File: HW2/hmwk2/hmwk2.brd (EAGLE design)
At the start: 50 x 50 mm, 22 parts, among them J1 USB_MINI-B_SMT

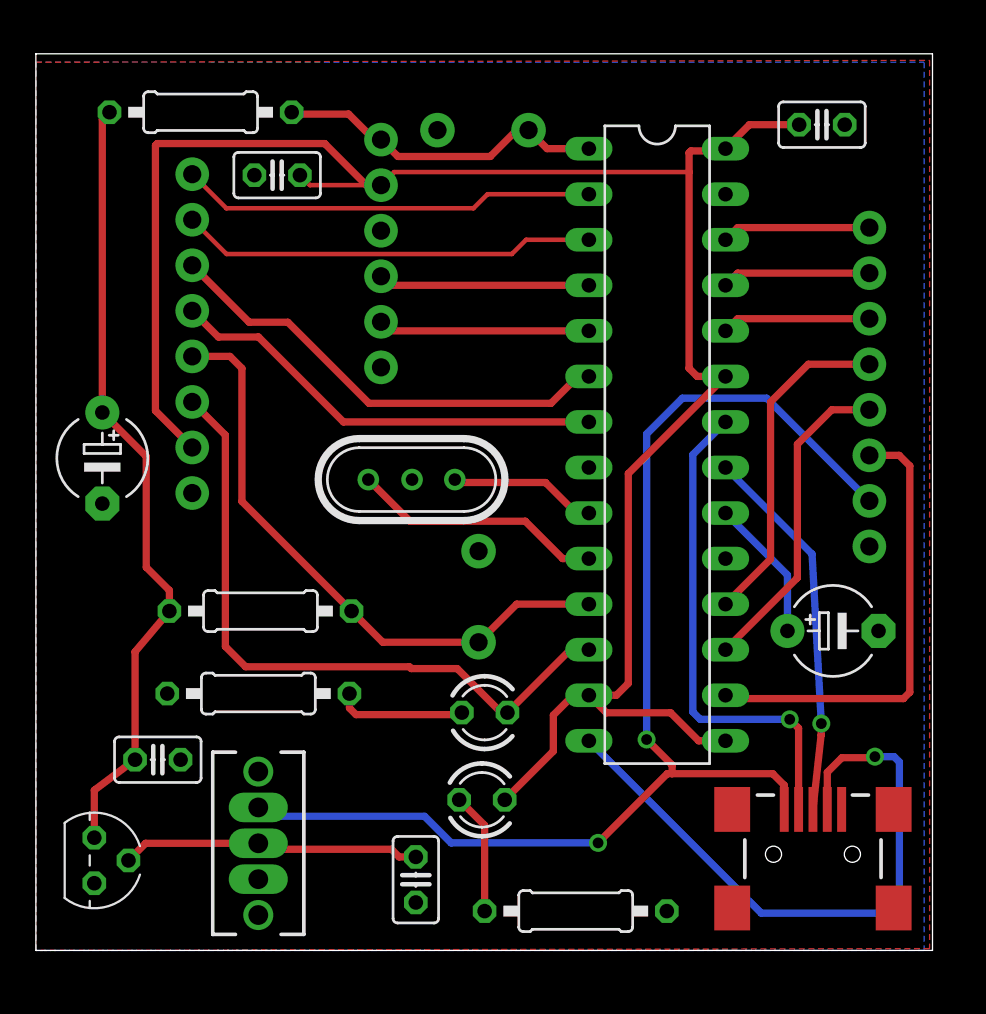
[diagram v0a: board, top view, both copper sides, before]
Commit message: updated board
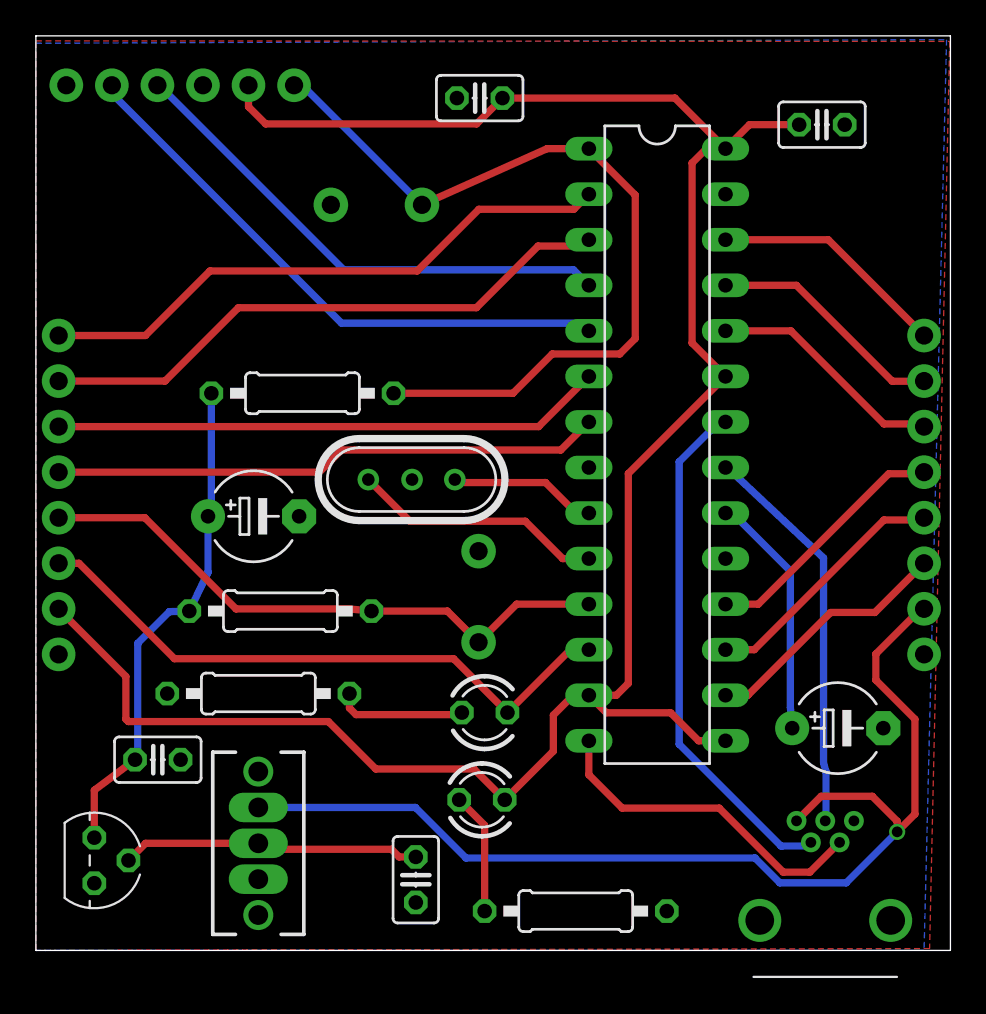
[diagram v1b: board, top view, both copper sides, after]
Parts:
- removed J1: USB_MINI-B_SMT, components:USB-MINIB
- added K1: 651005136521, components:651005136521
- moved J2 23.6 mm to (1.70, 48.2), turned to 180 degrees
- moved R1 16.7 mm to (14.9, 31.1)
- moved C5 12.1 mm to (24.7, 47.5)
- moved J3 11.7 mm to (1.27, 16.5)
- moved C3 9.04 mm to (12.1, 24.2), turned to 0 degrees
- moved U$2 7.26 mm to (19.0, 41.6)
- moved J4 6.75 mm to (49.5, 16.5)
- moved C2 5.43 mm to (44.7, 12.4)
- moved R3 1.11 mm to (13.6, 18.9)
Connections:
- net D+: now also K1.3; no longer J1.D+
- net D-: now also K1.2; no longer J1.D-
- net GND: now also K1.5; no longer J1.GND, J1.S1, J1.S2, J1.S3, J1.S4
- net ID: now also K1.4; no longer J1.ID
- net VIN: now also K1.1; no longer J1.VBUS
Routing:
- net MCLR: track 18.8 -> 46.3 mm
- net PGC: track 11.8 -> 32.5 mm
- net PGD: track 11.8 -> 28.7 mm
- net ID: track 35.6 -> 18.8 mm, vias 1 -> 0
- net +3V3: track 44.0 -> 28.1 mm
- net B7: track 25.6 -> 14.1 mm
- net A0: track 23.2 -> 32.8 mm
- net A1: track 23.2 -> 32.8 mm
- net VIN: track 68.5 -> 60.9 mm, vias 2 -> 1
- net B3: track 24.7 -> 30.7 mm
- net N$2: track 8.00 -> 13.7 mm
- net VDD: track 113.8 -> 119.0 mm
- net B14: track 8.30 -> 13.3 mm
- net B15: track 8.30 -> 13.3 mm
- net B13: track 8.30 -> 13.3 mm
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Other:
- board size 50 x 50 mm -> 51 x 51 mm
- board text added: "A0 A1 B2 B3 B4 A4 3.3V GND"
- board text removed: "A0 A1 B2 B3 B4"
- board text removed: "A4 3.3V GND"
